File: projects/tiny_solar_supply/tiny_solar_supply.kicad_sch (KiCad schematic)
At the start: 15 parts, among them J1 Conn_01x02, J2 Conn_01x02, J3 Conn_01x02, J4 Conn_01x02, Q1 2N7002

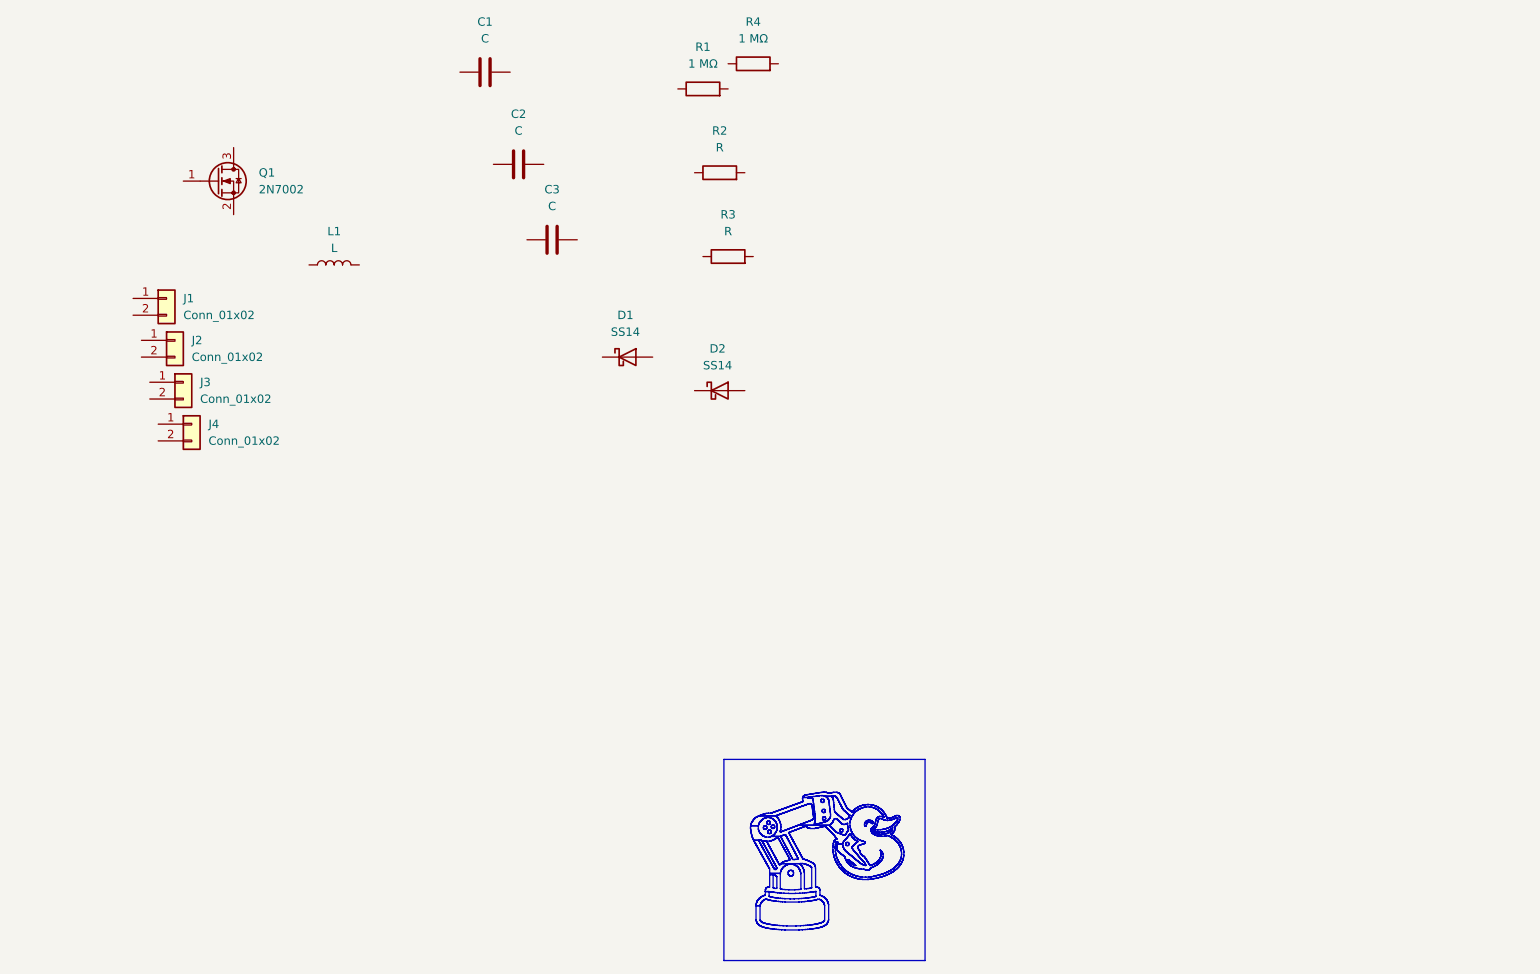
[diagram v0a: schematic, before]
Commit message: Initial commit of schematic
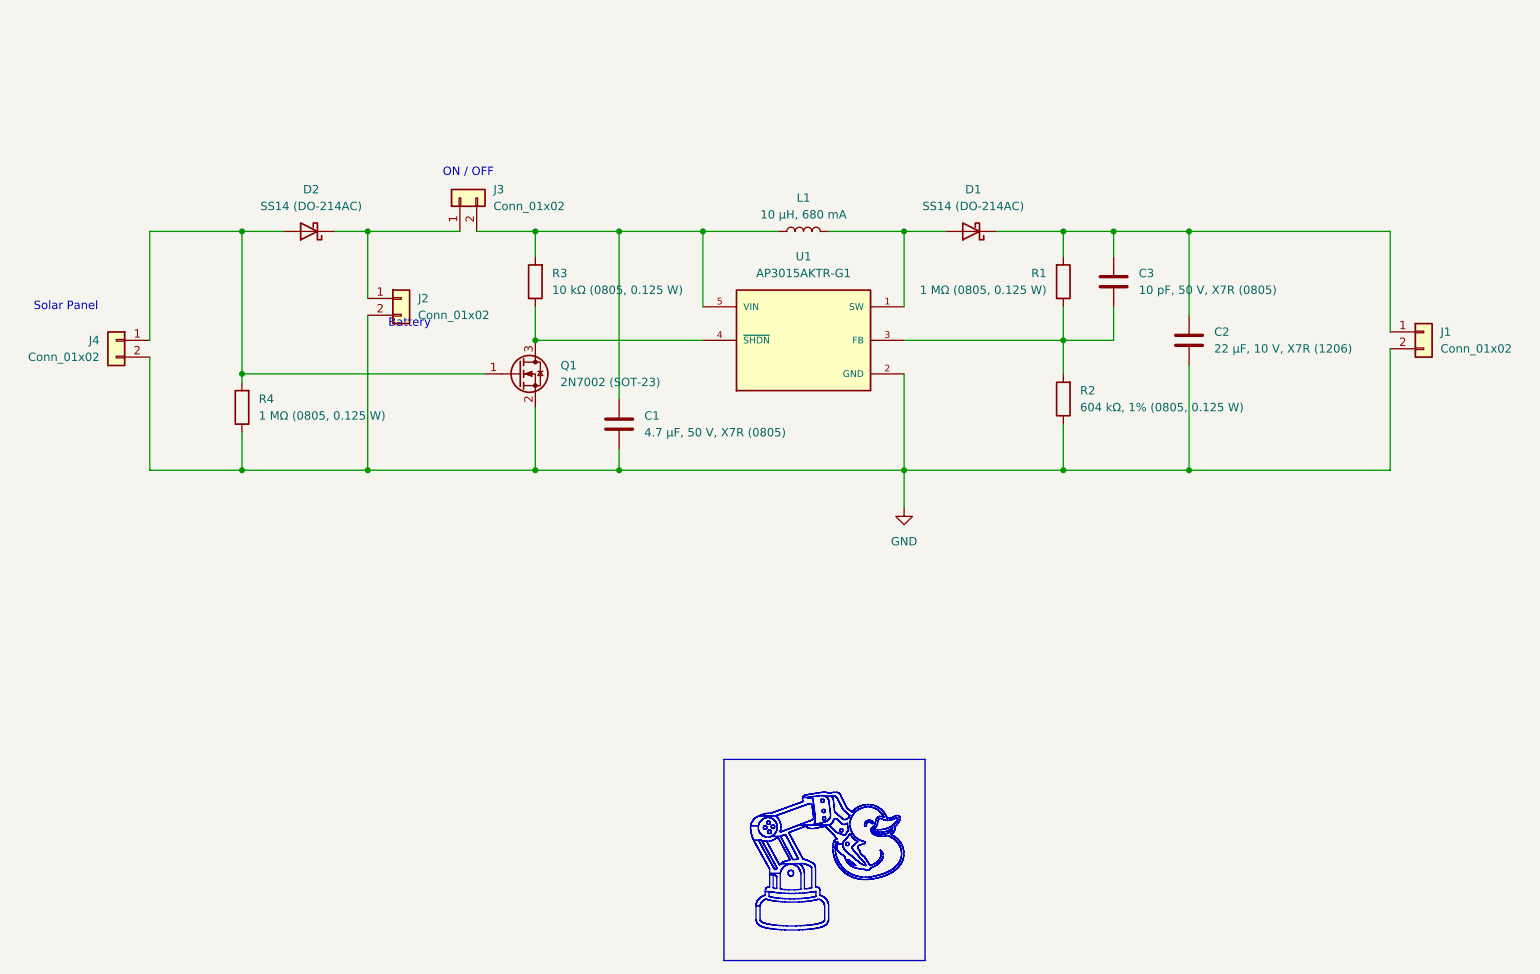
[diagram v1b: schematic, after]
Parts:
- removed J1, J2, J3, J4: Conn_01x02, symbol Connector_Generic:Conn_01x02
- added J1, J2, J3, J4: Conn_01x02, SparkFun-Connector:1x02, symbol SparkFun-Connector:Conn_01x02
- added U1: AP3015AKTR-G1, MH_AP3015A:SOT95P280X145-5N, symbol MH_AP3015A:AP3015AKTR-G1
- C1: value C -> 4.7 µF, 50 V, X7R (0805)
- C2: value C -> 22 µF, 10 V, X7R (1206)
- C3: value C -> 10 pF, 50 V, X7R (0805)
- D1, D2: value SS14 -> SS14 (DO-214AC); footprint Diode_SMD:D_SMA -> SparkFun-Semiconductor-Standard:SMA
- L1: value L -> 10 µH, 680 mA; footprint (none) -> MH_L1:IND_ASPI-0630LR_ABR
- Q1: value 2N7002 -> 2N7002 (SOT-23)
- R1, R4: value 1 MΩ -> 1 MΩ (0805, 0.125 W)
- R2: value R -> 604 kΩ, 1% (0805, 0.125 W)
- R3: value R -> 10 kΩ (0805, 0.125 W)
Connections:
- net GND: now reaches R4.1
- net GND: now also C1.1, C2.1, Q1.2 (S), R2.1, J1.2 (Pin_2), J2.2 (Pin_2), J4.2 (Pin_2), U1.2 (GND)
- net at R4.2: now also D2.2 (A), Q1.1 (G), J4.1 (Pin_1)
- net at L1.1: now also C1.2, R3.2, J3.2 (Pin_2), U1.5 (VIN)
- net at L1.2: now also D1.2 (A), U1.1 (SW)
- net at C2.2: now also C3.2, D1.1 (K), R1.2, J1.1 (Pin_1)
- net at R3.1: now also Q1.3 (D), U1.4 (~{SHDN})
- net at R1.1: now also C3.1, R2.2, U1.3 (FB)
- net at D2.1 (K): now also J2.1 (Pin_1), J3.1 (Pin_1)
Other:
- note added: "Battery"
- note added: "ON / OFF"
- note added: "Solar Panel"
- moved on the sheet: C1, C2, C3, D1, D2, L1, Q1, R1, R2, R3, R4

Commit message: Schematic - complete with ERC
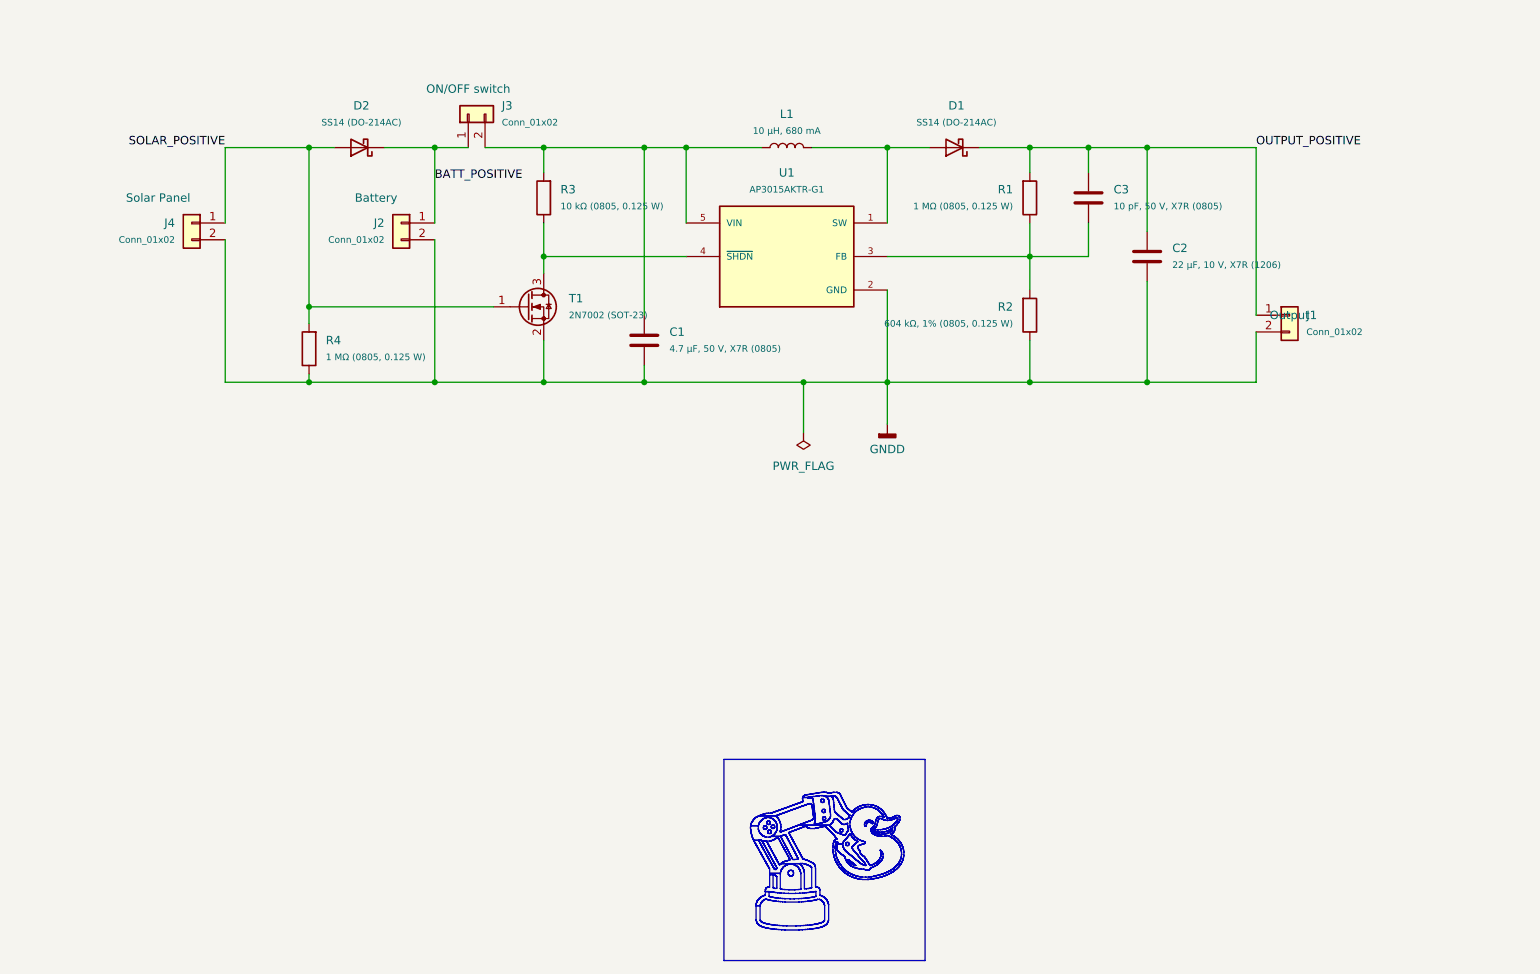
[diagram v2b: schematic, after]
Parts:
- J1: MH_Role (none) -> Output
- J2: MH_Role (none) -> Battery
- J3: MH_Role (none) -> ON/OFF switch
- J4: MH_Role (none) -> Solar Panel
- renumbered Q1 to T1
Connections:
- net SOLAR_POSITIVE: now reaches D2.2 (A), J4.1 (Pin_1), R4.2, T1.1 (G)
- net OUTPUT_POSITIVE: now reaches C2.2, C3.2, D1.1 (K), J1.1 (Pin_1), R1.2
- net BATT_POSITIVE: now reaches D2.1 (K), J2.1 (Pin_1), J3.1 (Pin_1)
- net GND renamed GNDD
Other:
- note removed: "Battery"
- note removed: "ON / OFF"
- note removed: "Solar Panel"
- moved on the sheet: C1, C2, C3, D1, D2, J1, J2, J3, J4, L1, R1, R2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
